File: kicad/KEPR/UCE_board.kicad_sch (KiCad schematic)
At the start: 13 parts, among them IC1 ACS37041KLHBLT-010B3, IC2 ACS37041KLHBLT-010B3, IC3 ACS37041KLHBLT-010B3, U1 REF193, U2 STM32G484CETx, U3 AMS1117-3.3

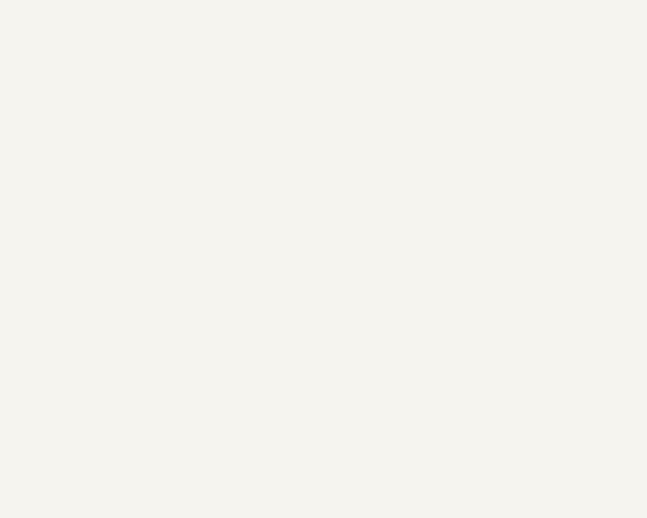
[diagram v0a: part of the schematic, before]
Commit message: mais ajustes de trilha.
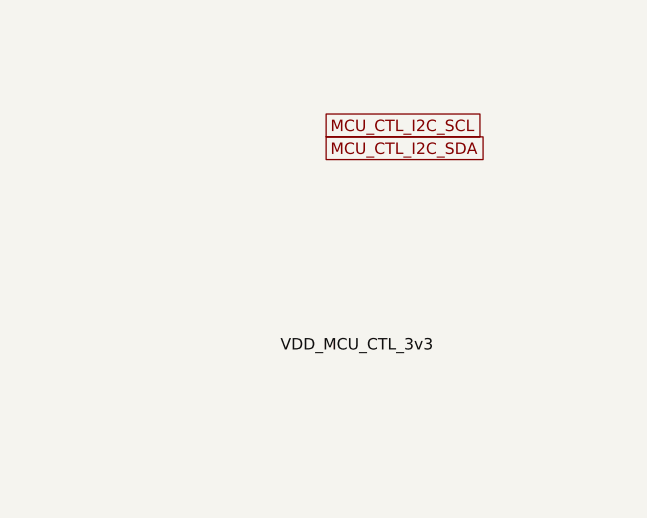
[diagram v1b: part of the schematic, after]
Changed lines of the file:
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@@
+		)
+	)
+	(label "VDD_MCU_CTL_3v3"
+		(at 323.85 54.61 0)
+		(effects
+			(font
+				(size 1.27 1.27)
+			)
+			(justify left bottom)
 		)
 	)
@@
 		)
 	)
+	(global_label "MCU_CTL_I2C_SCL"
+		(shape passive)
+		(at 328.93 29.21 0)
+		(fields_autoplaced yes)
+		(effects
+			(font
+				(size 1.27 1.27)
+			)
+			(justify left)
+		)
+		(property "Intersheetrefs" "${INTERSHEET_REFS}"
+			(at 347.6162 29.21 0)
+			(effects
+				(font
+					(size 1.27 1.27)
+				)
+				(justify left)
+				(hide yes)
+			)
+		)
+	)
 	(global_label "+12v Shunt"
 		(shape input)
@@
 			)
 		)
+	)
+	(global_label "MCU_CTL_I2C_SDA"
+		(shape passive)
+		(at 328.93 31.75 0)
+		(fields_autoplaced yes)
+		(effects
+			(font
+				(size 1.27 1.27)
+			)
+			(justify left)
+		)
+		(property "Intersheetrefs" "${INTERSHEET_REFS}"
+			(at 347.6767 31.75 0)
+			(effects
+				(font
+					(size 1.27 1.27)
+				)
+				(justify left)
+				(hide yes)
+			)
+		)
+	)
+	(rule_area
+		(polyline
+			(pts
+				(xy 350.52 25.4) (xy 350.52 38.1) (xy 345.44 38.1) (xy 317.5 38.1) (xy 317.5 25.4) (xy 317.5 25.4)
+			)
+			(stroke
+				(width 0)
+				(type dash)
+			)
+			(fill
+				(type none)
+			)
+		)
+	)
+	(rule_area
+		(polyline
+			(pts
+				(xy 317.5 49.53) (xy 350.52 49.53) (xy 350.52 63.5) (xy 317.5 63.5)
+			)
+			(stroke
+				(width 0)
+				(type dash)
+			)
+			(fill
+				(type none)
+			)
+		)
+	)
+	(netclass_flag ""
+		(length 2.54)
+		(shape round)
+		(at 326.39 49.53 0)
+		(fields_autoplaced yes)
+		(effects
+			(font
+				(size 1.27 1.27)
+			)
+			(justify left bottom)
+		)
+		(property "Netclass" "VDD_MCU_CTL"
+			(at 327.0885 46.99 0)
+			(effects
+				(font
+					(size 1.27 1.27)
+				)
+				(justify left)
+			)
+		)
+		(property "Component Class" ""
+			(at -87.63 -8.89 0)
+			(effects
+				(font
+					(size 1.27 1.27)
+					(italic yes)
+				)
+			)
+		)
+	)
+	(netclass_flag ""
+		(length 2.54)
+		(shape round)
+		(at 331.47 25.4 0)
+		(fields_autoplaced yes)
+		(effects
+			(font
+				(size 1.27 1.27)
+			)
+			(justify left bottom)
+		)
+		(property "Netclass" "I2C"
+			(at 332.1685 22.86 0)
+			(effects
+				(font
+					(size 1.27 1.27)
+				)
+				(justify left)
+			)
+		)
+		(property "Component Class" ""
+			(at -113.03 -27.94 0)
+			(effects
+				(font
+					(size 1.27 1.27)
+					(italic yes)
+				)
+			)
+		)
